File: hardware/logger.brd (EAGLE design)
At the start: 33.5 x 32.9 mm, 40 parts, among them J1 MICRO_USB_B_HIROSE_ZX62-B-5PA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, SW1 TVAF06-A020B-R, U2 NJM12888F, X1 FA-238

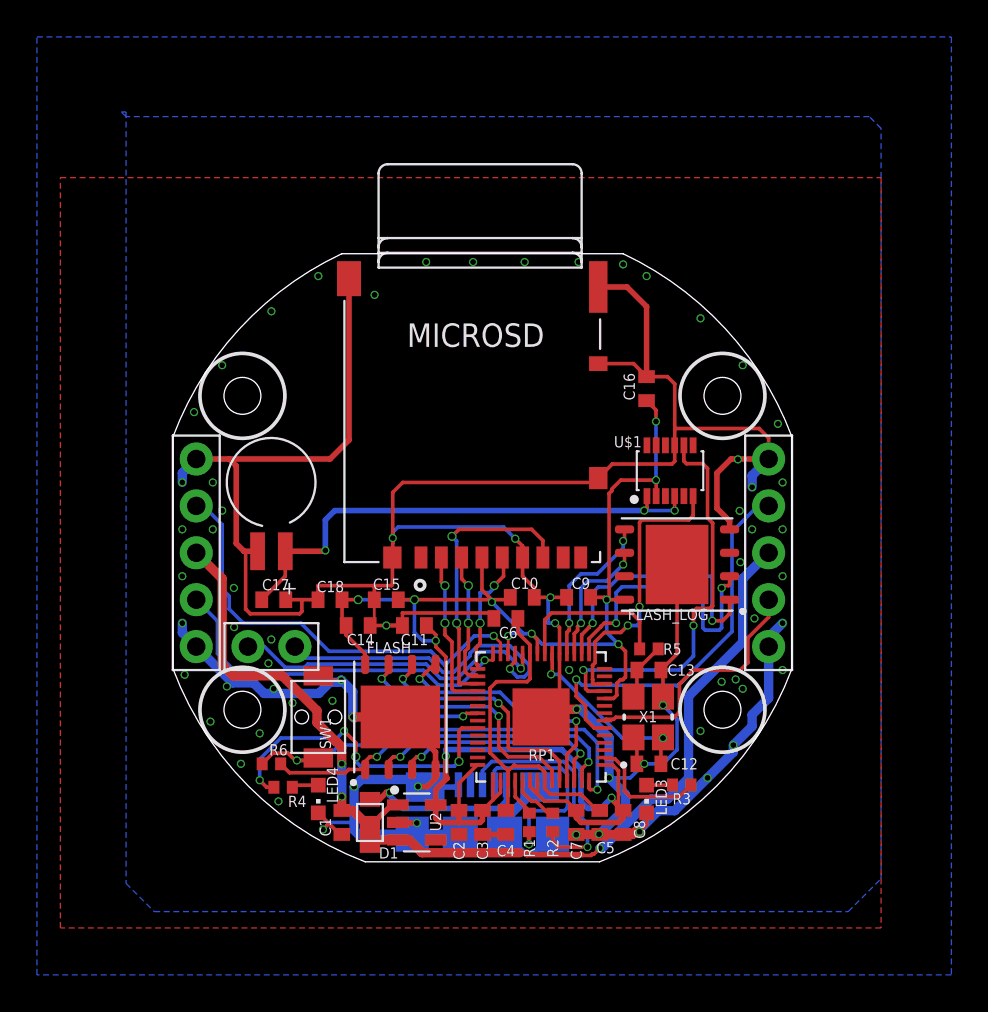
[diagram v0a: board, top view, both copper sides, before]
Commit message: 微修正
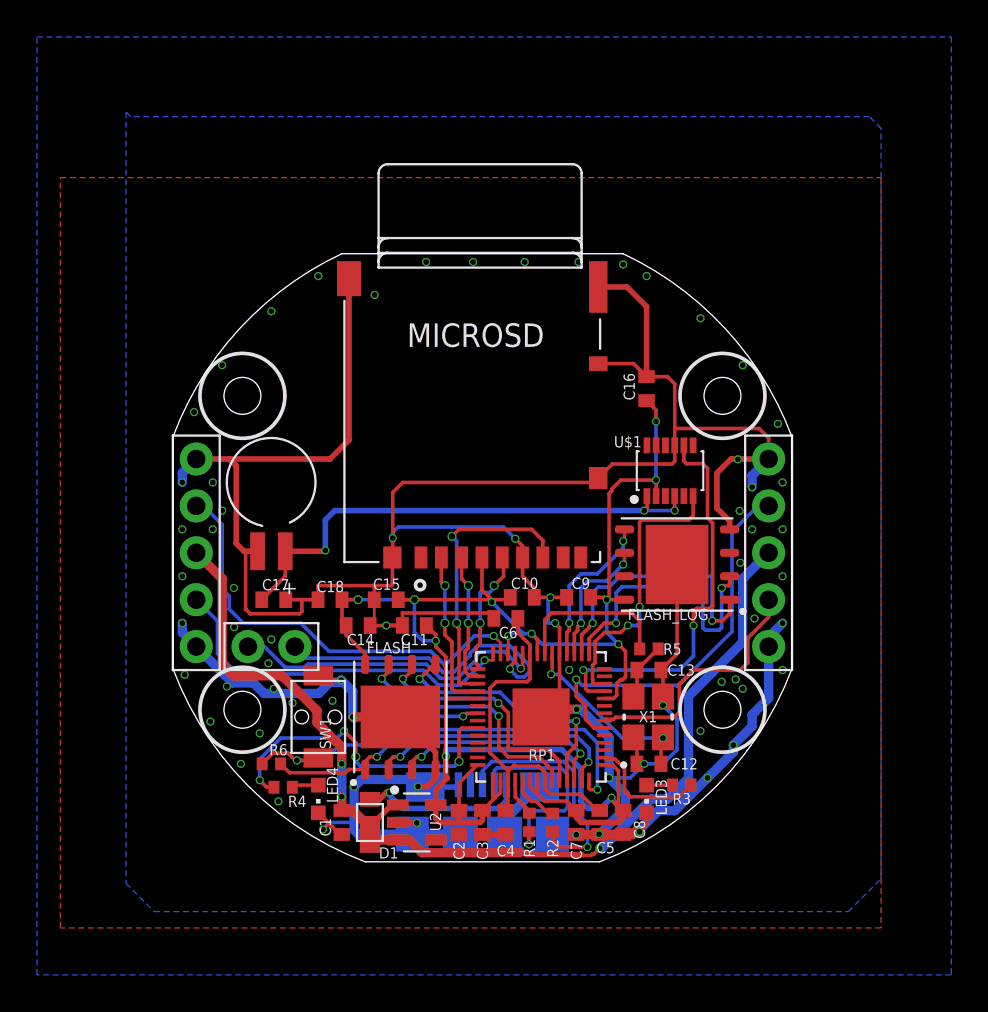
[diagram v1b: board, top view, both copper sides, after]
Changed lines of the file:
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@@
 <via x="14.605" y="3.556" extent="1-16" drill="0.3"/>
 <via x="14.605" y="1.27" extent="1-16" drill="0.3"/>
-<via x="13.97" y="-0.508" extent="1-16" drill="0.3"/>
+<via x="13.97" y="-0.5395" extent="1-16" drill="0.3"/>
 <via x="14.732" y="-3.556" extent="1-16" drill="0.3"/>
 <via x="13.716" y="-6.858" extent="1-16" drill="0.3"/>
@@
 <wire x1="-9.906" y1="-3.302" x2="-9.779" y2="-3.175" width="0.2" layer="1"/>
 <wire x1="-9.779" y1="-3.175" x2="-9.779" y2="-2.54" width="0.2" layer="1"/>
-<wire x1="-4.8585" y1="0.7965" x2="-4.8585" y2="0.508" width="0.2" layer="1"/>
-<wire x1="-4.8585" y1="0.508" x2="-4.8585" y2="-0.3625" width="0.2" layer="1"/>
+<wire x1="-4.8585" y1="0.7965" x2="-4.8585" y2="-0.3625" width="0.2" layer="1"/>
 <wire x1="-4.8585" y1="-0.3625" x2="-4.877" y2="-0.381" width="0.2" layer="1"/>
 <wire x1="1.778" y1="0.762" x2="2.173" y2="0.367" width="0.2" layer="1"/>
@@
 <vertex x="21.59" y="22.987"/>
 <vertex x="20.955" y="23.622"/>
-<vertex x="-19.304" y="23.622"/>
-<vertex x="-19.558" y="23.876"/>
+<vertex x="-19.05" y="23.622"/>
 </polygon>
-<wire x1="11.811" y1="12.7" x2="14.097" y2="10.16" width="0" layer="19" extent="1-1"/>
-<wire x1="16.002" y1="6.985" x2="14.097" y2="10.16" width="0" layer="19" extent="1-1"/>
-<wire x1="15.5" y1="5.08" x2="16.002" y2="6.985" width="0" layer="19" extent="1-1"/>
-<wire x1="6.35" y1="-15.255" x2="6.3165" y2="-15.241" width="0" layer="19" extent="1-1"/>
-<wire x1="-1.27" y1="-15.255" x2="-1.2" y2="-15.24" width="0" layer="19" extent="1-16"/>
-<wire x1="1.27" y1="-15.255" x2="1.2" y2="-15.24" width="0" layer="19" extent="1-16"/>
-<wire x1="-3.49" y1="-12.6605" x2="-3.1" y2="-12.69" width="0" layer="19" extent="16-16"/>
-<wire x1="-8.124" y1="-8.0145" x2="-7.678" y2="-6.9595" width="0" layer="19" extent="16-16"/>
-<wire x1="13.933" y1="2.273" x2="13.386" y2="1.27" width="0" layer="19" extent="1-1"/>
-<wire x1="14.605" y1="1.27" x2="13.386" y2="1.27" width="0" layer="19" extent="1-1"/>
-<wire x1="16.256" y1="3.81" x2="15.5" y2="5.08" width="0" layer="19" extent="1-1"/>
-<wire x1="16.256" y1="-6.35" x2="15.5" y2="-5.08" width="0" layer="19" extent="1-1"/>
-<wire x1="14.732" y1="-3.556" x2="16.256" y2="-3.81" width="0" layer="19" extent="1-1"/>
-<wire x1="-14.605" y1="3.81" x2="-15.5" y2="5.08" width="0" layer="19" extent="1-1"/>
-<wire x1="-14.097" y1="2.286" x2="-14.605" y2="3.81" width="0" layer="19" extent="1-1"/>
-<wire x1="-14.605" y1="1.27" x2="-14.097" y2="2.286" width="0" layer="19" extent="1-1"/>
-<wire x1="-16.129" y1="-6.604" x2="-15.5" y2="-5.08" width="0" layer="19" extent="1-1"/>
-<wire x1="-16.256" y1="1.27" x2="-14.605" y2="1.27" width="0" layer="19" extent="1-1"/>
-<wire x1="16.256" y1="1.27" x2="14.605" y2="1.27" width="0" layer="19" extent="1-1"/>
-<wire x1="13.8385" y1="5.0585" x2="15.5" y2="5.08" width="0" layer="19" extent="1-1"/>
-<wire x1="-5.842" y1="13.97" x2="-7.227" y2="14.846" width="0" layer="19" extent="1-1"/>
-<wire x1="-8.89" y1="14.986" x2="-7.227" y2="14.846" width="0" layer="19" extent="1-1"/>
-<wire x1="5.207" y1="15.748" x2="6.273" y2="14.396" width="0" layer="19" extent="1-1"/>
-<wire x1="7.62" y1="15.621" x2="6.273" y2="14.396" width="0" layer="19" extent="1-1"/>
-<wire x1="8.89" y1="14.986" x2="7.62" y2="15.621" width="0" layer="19" extent="1-1"/>
-<wire x1="13.97" y1="-0.508" x2="13.386" y2="1.27" width="0" layer="19" extent="1-1"/>
-<wire x1="11.811" y1="-9.652" x2="13.589" y2="-10.414" width="0" layer="19" extent="1-1"/>
-<wire x1="-10.287" y1="-8.128" x2="-8.89" y2="-6.665" width="0" layer="19" extent="1-1"/>
-<wire x1="-11.303" y1="-7.366" x2="-10.287" y2="-8.128" width="0" layer="19" extent="1-1"/>
-<wire x1="-11.592" y1="-5.985" x2="-11.303" y2="-7.366" width="0" layer="19" extent="1-1"/>
-<wire x1="-11.4345" y1="-4.6935" x2="-11.592" y2="-5.985" width="0" layer="19" extent="1-1"/>
-<wire x1="-13.45" y1="-4.0235" x2="-11.4345" y2="-4.6935" width="0" layer="19" extent="1-1"/>
-<wire x1="-13.462" y1="-1.905" x2="-13.45" y2="-4.0235" width="0" layer="19" extent="1-1"/>
-<wire x1="-11.049" y1="-13.462" x2="-8.89" y2="-14.085" width="0" layer="19" extent="1-1"/>
-<wire x1="-13.843" y1="-7.239" x2="-16.129" y2="-6.604" width="0" layer="19" extent="1-1"/>
-<wire x1="-14.732" y1="-9.144" x2="-13.843" y2="-7.239" width="0" layer="19" extent="1-1"/>
-<wire x1="14.097" y1="-7.366" x2="16.256" y2="-6.35" width="0" layer="19" extent="1-1"/>
-<wire x1="13.716" y1="-6.858" x2="14.097" y2="-7.366" width="0" layer="19" extent="1-1"/>
-<wire x1="12.954" y1="-6.985" x2="13.716" y2="-6.858" width="0" layer="19" extent="1-1"/>
-<wire x1="-12.065" y1="-9.779" x2="-10.287" y2="-8.128" width="0" layer="19" extent="1-1"/>
-<wire x1="-13.081" y1="-11.43" x2="-12.065" y2="-9.779" width="0" layer="19" extent="1-1"/>
-<wire x1="16.256" y1="-1.27" x2="13.97" y2="-0.508" width="0" layer="19" extent="1-1"/>
-<wire x1="-16.256" y1="-1.27" x2="-16.256" y2="-3.81" width="0" layer="19" extent="1-1"/>
-<wire x1="-15.621" y1="7.62" x2="-15.5" y2="5.08" width="0" layer="19" extent="1-1"/>
-<wire x1="2.286" y1="15.748" x2="5.207" y2="15.748" width="0" layer="19" extent="1-1"/>
-<wire x1="-0.508" y1="15.748" x2="2.286" y2="15.748" width="0" layer="19" extent="1-1"/>
-<wire x1="-3.048" y1="15.748" x2="-0.508" y2="15.748" width="0" layer="19" extent="1-1"/>
-<wire x1="-14.097" y1="10.16" x2="-15.621" y2="7.62" width="0" layer="19" extent="1-1"/>
-<wire x1="-11.43" y1="13.081" x2="-8.89" y2="14.986" width="0" layer="19" extent="1-1"/>
 </signal>
 <signal name="USB_DM">
